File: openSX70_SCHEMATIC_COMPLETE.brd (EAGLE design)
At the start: 95.9 x 27.9 mm, 41 parts, among them Q1 5.8A/30V/35mΩ, Q2 5.8A/30V/35mΩ, U1 ATMEGA328P_TQFP, U3 BH1750FVI-TR, Y1 16MHz

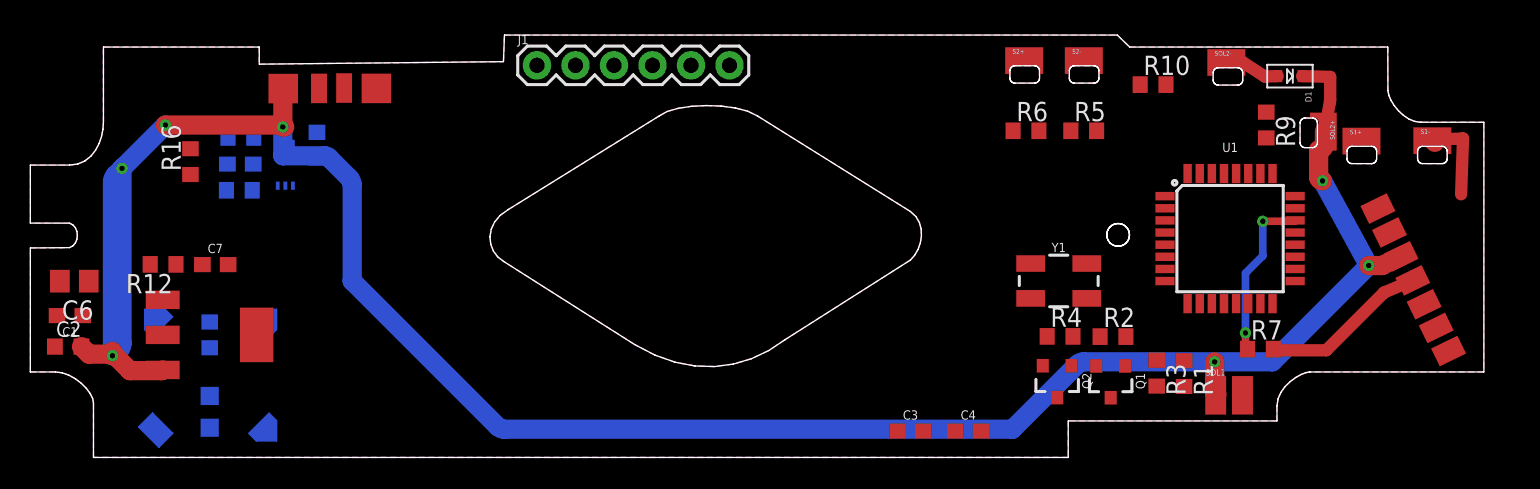
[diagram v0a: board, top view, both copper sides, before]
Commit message: Eagle openSX70 pcb layout 2.0
Layout 2.0
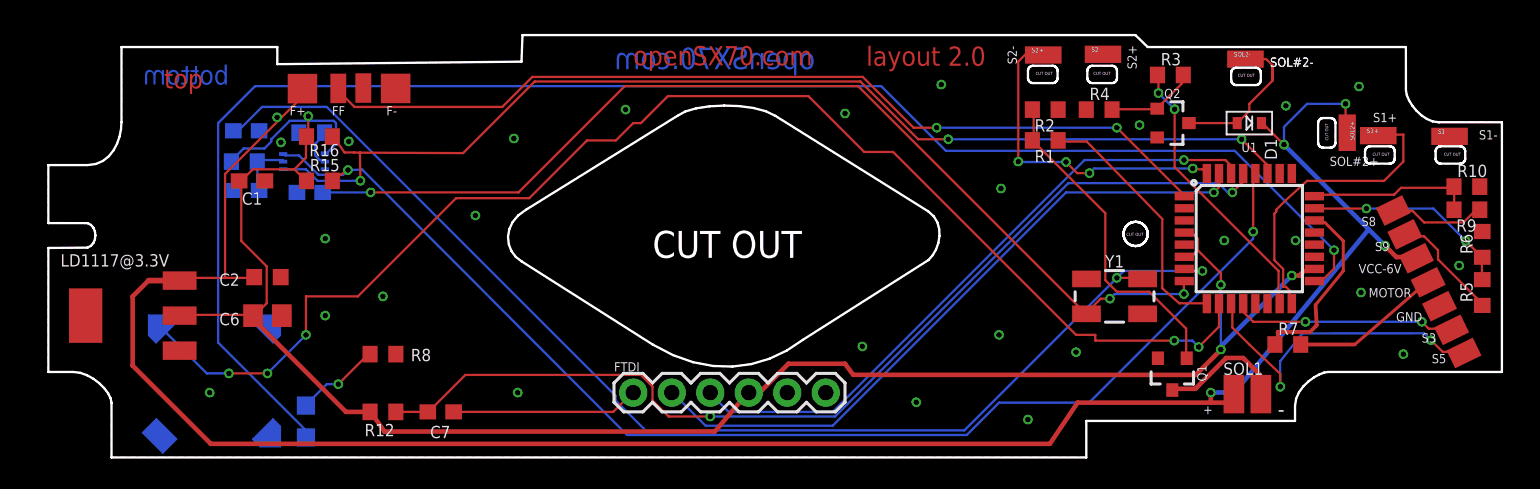
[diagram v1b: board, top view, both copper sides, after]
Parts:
- removed BUZZ1: CSET8-5G, CSET8-5G_B:CSET8-5G_PACKAGE
- removed J1: (no value), SparkFun-Connectors:1X06
- removed U3: BH1750FVI-TR, openSX70:SOTFL50P300X75-6N
- added BH1750: BH1750FVI-TR, openSX70:SOTFL50P300X75-6N
- added BUZZER: CSET8-5G, CSET8-5G_B:CSET8-5G_PACKAGE
- added FTDI: FTDI HEADER, SparkFun-Connectors:1X06
- S1+, S1-, S2+, S2-, SOL2+, SOL2-: value SX70_S-PAD -> SX70-S-PAD-NEW; device openSX70:SX70-S-PAD -> openSX70:SX70-S-PAD2
- moved C4 51.6 mm to (15.1, 22.4), flipped to the bottom
- moved C3 42.6 mm to (19.3, 18.3), flipped to the bottom, turned to 180 degrees
- moved R6 31.0 mm to (96.6, 14.9), turned to 90 degrees
- moved R5 28.4 mm to (96.6, 11.7), turned to 90 degrees
- moved R10 21.8 mm to (95.6, 18.7)
- moved R3 19.7 mm to (76.1, 26.0), turned to 0 degrees
- moved Q2 18.6 mm to (76.2, 22.9), turned to 270 degrees
- moved R1 17.9 mm to (67.8, 21.7), turned to 180 degrees
- moved C7 17.8 mm to (27.9, 3.81), turned to 180 degrees
- moved R12 17.5 mm to (24.1, 3.81)
- moved R2 15.6 mm to (67.8, 23.7), turned to 180 degrees
- moved R4 15.2 mm to (71.4, 23.7)
- moved C1 14.9 mm to (15.5, 19.1)
- moved R9 14.4 mm to (95.6, 17.1), turned to 180 degrees
- moved C2 13.9 mm to (16.5, 12.7), turned to 180 degrees
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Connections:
- removed net N$9 (its old number): C5.1, R13.1, U3.5
- new net N$2: BH1750.5, C5.1, R13.1
- net 3.3V: now also BH1750.1, FTDI.4; no longer J1.4, U3.1
- net BUZZER: now also BUZZER.+
- net DTR: now also FTDI.1; no longer J1.1
- net GND: now also BH1750.3, BUZZER.GND-, FTDI.6; no longer J1.6, U3.3
- net N$10: now also BH1750.2; no longer U3.2
- net RXD: now also FTDI.3; no longer J1.3
- net SCL: now also BH1750.6; no longer U3.6
- net SDA: now also BH1750.4; no longer U3.4
- net TXD: now also FTDI.2; no longer J1.2
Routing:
- net 3.3V: track 0.00 -> 123.8 mm, vias 0 -> 4
- net LED: track 0.00 -> 105.1 mm, vias 0 -> 1
- net BUZZER: track 0.00 -> 89.1 mm, vias 0 -> 5
- net SCL: track 0.00 -> 83.0 mm, vias 0 -> 2
- net N$4: track 0.00 -> 80.9 mm, vias 0 -> 2
- net SDA: track 0.00 -> 74.3 mm, vias 0 -> 3
- net N$6: track 0.00 -> 67.4 mm, vias 0 -> 3
- net N$9: track 0.00 -> 66.1 mm, vias 0 -> 2
- net FF: track 0.00 -> 60.5 mm, vias 0 -> 2
- net TXD: track 0.00 -> 44.4 mm, vias 0 -> 1
- net RXD: track 0.00 -> 42.5 mm, vias 0 -> 1
- net N$11: track 24.5 -> 0.00 mm, vias 2 -> 0
- net 6V: track 119.4 -> 142.3 mm
- net S5: track 0.00 -> 22.1 mm, vias 0 -> 2
- net N$1: track 0.00 -> 21.9 mm
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- added copper zone on layer 1, net N$11
- added copper zone on layer 1, net N$12
- added copper zone on layer 1, net N$13
- added copper zone on layer 1, net N$14
- added copper zone on layer 1, net N$16
- added copper zone on layer 1, net N$17
- added copper zone on layer 16, net N$18
- added copper zone on layer 16, net N$19
- added copper zone on layer 16, net N$20
- added copper zone on layer 16, net N$21
- added copper zone on layer 16, net N$22
- added copper zone on layer 16, net N$23
- added copper zone on layer 16, net N$24
- added copper zone on layer 16, net N$25
- added copper zone on layer 1, net N$7
- added copper zone on layer 1, net N$8
- removed copper zone on layer 16, net S$11
- removed copper zone on layer 16, net S$12
- removed copper zone on layer 16, net S$13
- removed copper zone on layer 16, net S$14
- removed copper zone on layer 16, net S$15
- removed copper zone on layer 16, net S$16
- removed copper zone on layer 16, net S$17
- removed copper zone on layer 16, net S$18
- removed copper zone on layer 1, net S$2
- removed copper zone on layer 1, net S$3
- removed copper zone on layer 1, net S$4
- removed copper zone on layer 1, net S$5
- removed copper zone on layer 1, net S$6
- removed copper zone on layer 1, net S$7
- removed copper zone on layer 1, net S$8
- removed copper zone on layer 1, net S$9
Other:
- outline, holes or cut-outs redrawn
- board text added: "+"
- board text added: "-"
- board text added: "CUT OUT"
- board text added: "F+"
- board text added: "F-"
- board text added: "FF"
- board text added: "GND"
- board text added: "LD1117@3.3V"
- board text added: "MOTOR"
- board text added: "S1+"
- board text added: "S1-"
- board text added: "S2+"
- board text added: "S2-"
- board text added: "S3"
- board text added: "S5"
- board text added: "S8"
- board text added: "S9"
- board text added: "SOL#2+"
- board text added: "SOL#2-"
- board text added: "VCC-6V"
- board text added: "bottom"
- board text added: "layout 2.0"
- board text added: "openSX70.com"
- board text added: "top"
